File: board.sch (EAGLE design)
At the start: 75 parts, among them IC1 LM1117, J1 LHBEAMOUT, J10 ATEMP, J11 HORNOUT, J12 12V_SUPPLY, J13 STOPOUT, J14 TURNOUT, J15 FANOUT, J16 BLIGHTOUT, J17 AUXOUT, J18 AUX, J19 CAN, J2 BATT, J3 BLIGHT, J4 LHBEAM, J5 LRTURN, J6 WARNING, J7 HORN, J8 BREAK, J9 ABREAK, Q1 IRF7465TR, Q2 IRF7465TR, Q3 IRF7465TR, Q4 IRLML9301TRPBF, Q5 IRLML9301TRPBF, Q6 IRF7424TRPBF, Q7 IRF7424TRPBF, Q8 IRF7424TRPBF, Q9 IRLML9301TRPBF, U1 VOM1271T, U2 VOM1271T, U3 VOM1271T, U4 MC14504BDR2G, U5 MAX3051ESA+T

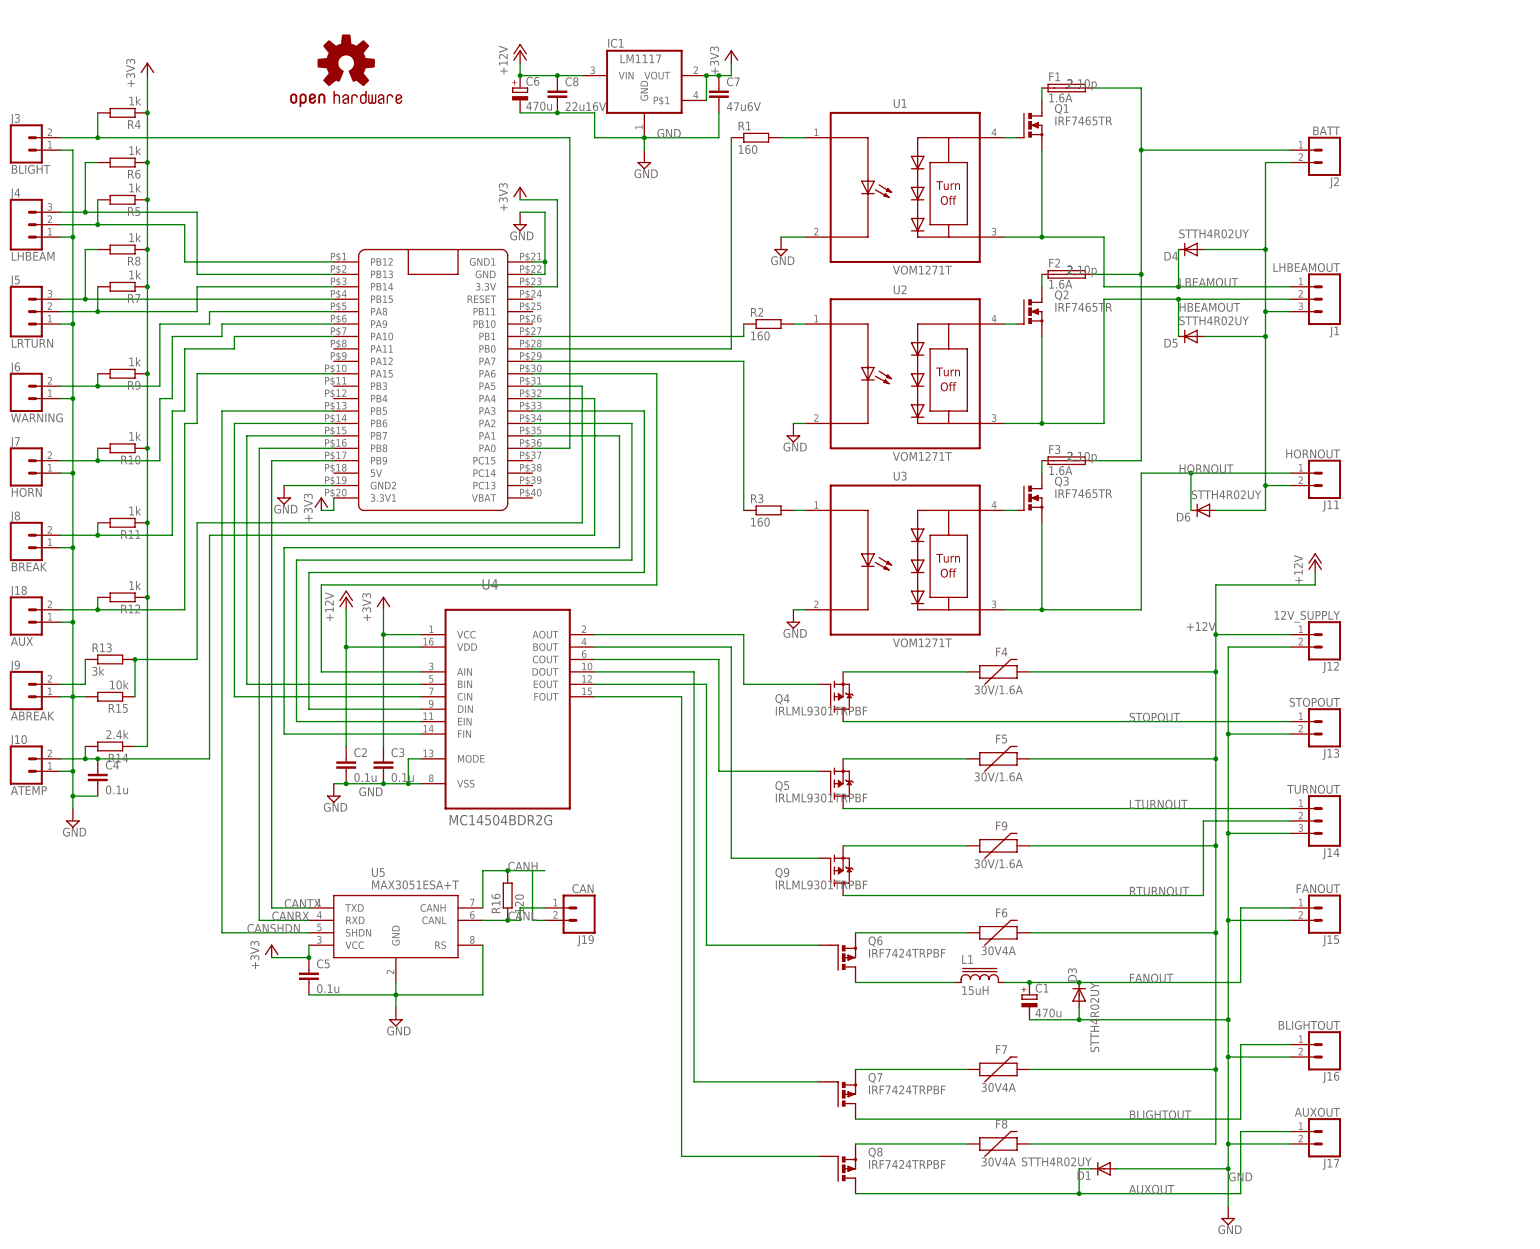
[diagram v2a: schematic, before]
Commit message: WIP
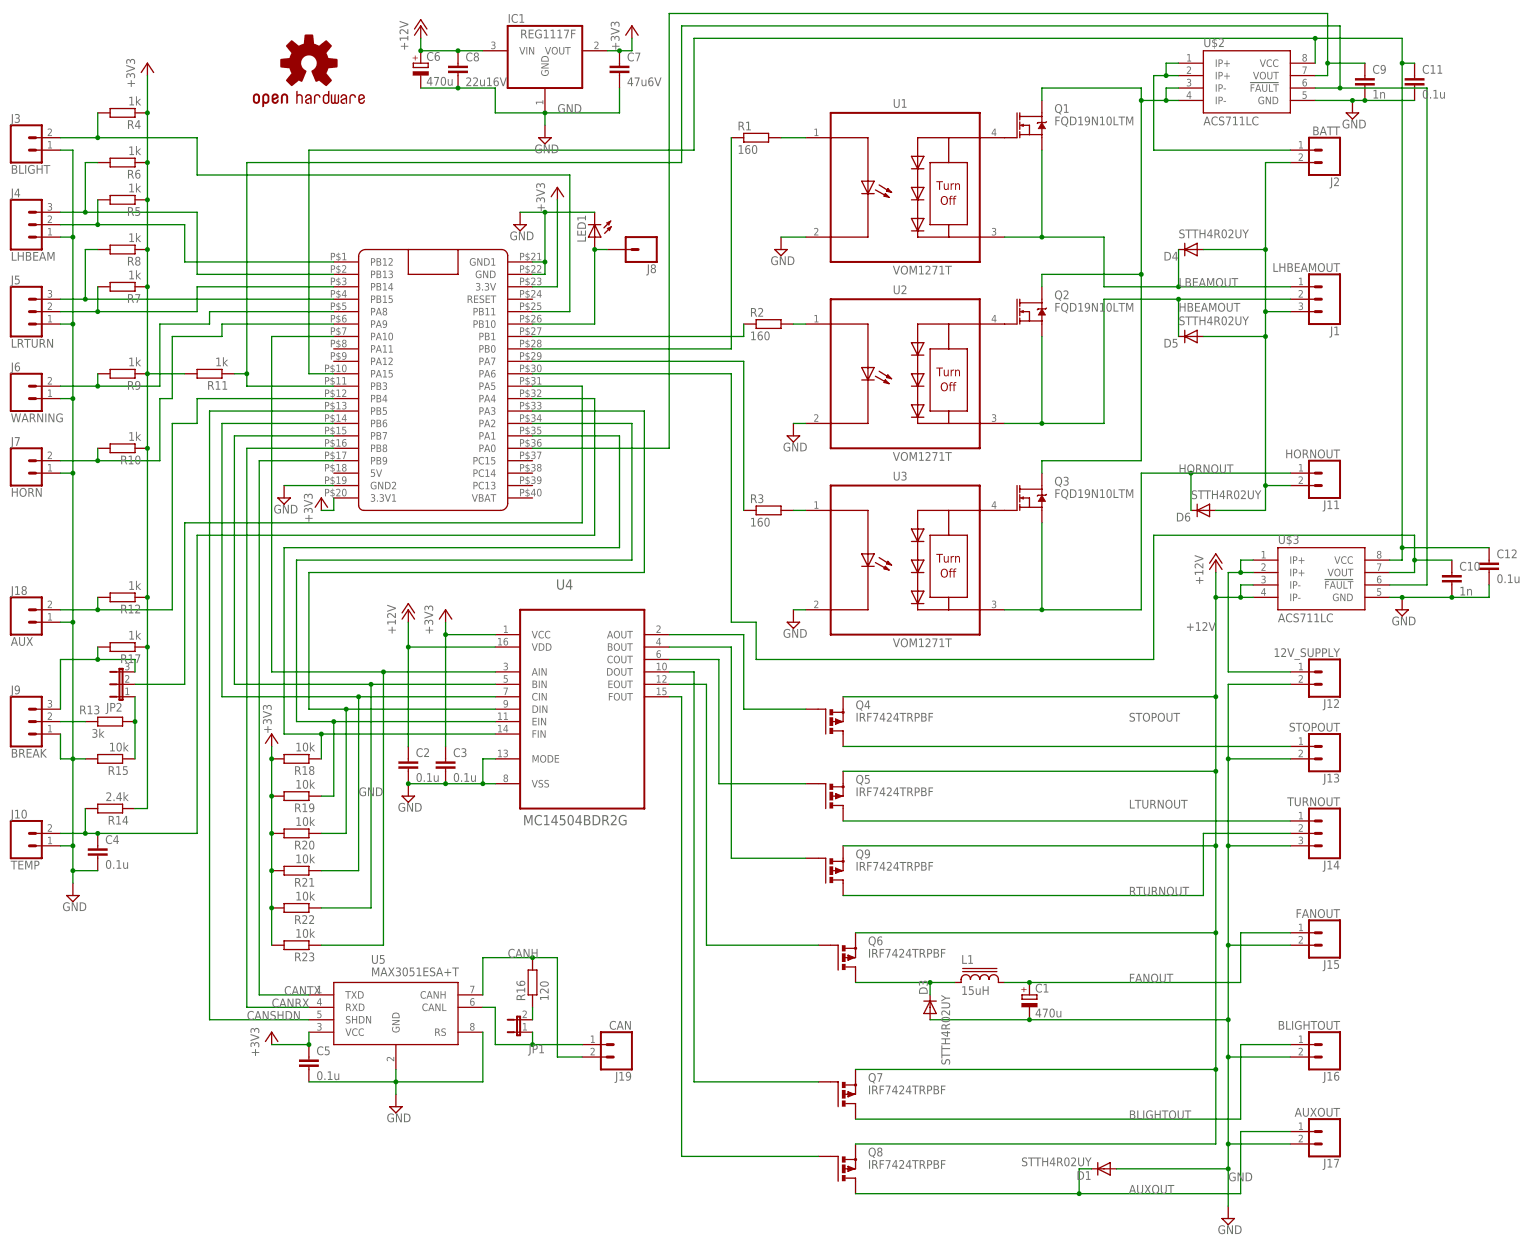
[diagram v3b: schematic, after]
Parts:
- removed F1, F2, F3: 1.6A, fuse:SHK20L
- removed F4, F5, F9: 30V/1.6A, SparkFun-Fuses:PPTC_PTH
- removed F6, F7, F8: 30V4A, svetozar:PPTC_WIDE
- added C10, C9: 1n, rcl:C-EUC0805
- added C11, C12: 0.1u, rcl:C-EUC0805
- added JP1: (no value), jumper:JP1E
- added JP2: (no value), jumper:JP2E
- added LED1: (no value), led:LEDSML0805
- added R17: 1k, rcl:R-EU_R0603
- added R18, R19, R20, R21, R22, R23: 10k, rcl:R-EU_R0603
- added U$2, U$3: ACS711LC, svetozar:ACS711
- C1, C6: device rcl:CPOL-EUE3.5-8 -> rcl:CPOL-EUF
- IC1: value LM1117 -> REG1117F; device svetozar:LM1117 -> burr-brown:REG1117F
- J10: value ATEMP -> TEMP
- J8: value BREAK -> (none); device SparkFun-Connectors:CONN_023.5MM -> SparkFun-Connectors:CONN_01; MPN DG350-3.5-02P-14-00AH -> (none); PRICE 5,80р -> (none); SHOP https://www.terraelectronica.ru/product/1115132 -> (none)
- J9: value ABREAK -> BREAK; device SparkFun-Connectors:CONN_023.5MM -> SparkFun-Connectors:CONN_03SCREW
- Q1, Q2, Q3: value IRF7465TR -> FQD19N10LTM; device transistor-power:N-MOSFET-SO8S -> SparkFun-DiscreteSemi:MOSFET-NCH-FDD8780; MPN IRF7465TRPBF -> FQD19N10LTM; PRICE 26,30р -> 15,80р; SHOP https://www.terraelectronica.ru/product/507651 -> https://www.terraelectronica.ru/product/675613
- Q4: value IRLML9301TRPBF -> IRF7424TRPBF; device svetozar:IRLML9301TRPBF -> transistor-power:P-MOSFET-SO8
- Q5, Q9: value IRLML9301TRPBF -> IRF7424TRPBF; device my:IRLML9301TRPBF -> transistor-power:P-MOSFET-SO8
- R10, R12, R13, R14, R15, R4, R5, R6, R7, R8, R9: device rcl:R-EU_R0805 -> rcl:R-EU_R0603
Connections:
- net ABRK renamed N$5
- removed net CANL: J19.1, R16.1, U5.CANL
- removed net HV1: F1.1A, Q1.D
- removed net HV2: F2.1A, Q2.D
- removed net HV3: F3.1A, Q3.D
- removed net N$15: J3.2, R4.2, U$1.PA0
- removed net N$16: F4.1, Q4.S
- removed net N$18: F5.1, Q5.S
- removed net N$19: F6.1, Q6.S
- removed net N$21: F7.1, Q7.S
- removed net N$22: F8.1, Q8.S
- removed net N$23: F9.1, Q9.S
- removed net N$34: J8.2, R11.2, U$1.PA10
- removed net N$36: J18.2, R12.2, U$1.PA15
- new net BATT+IN: J2.1, U$2.IP+@1, U$2.IP+@2
- new net CSENS1: C9.1, U$1.PA0, U$2.VOUT
- new net FAULT: R11.1, U$1.PB3, U$2.!FAULT, U$3.!FAULT
- new net IAUX: J18.2, R12.2, U$1.PB4
- new net IBLGHT: J3.2, R4.2, U$1.PB11
- new net N$1: JP1.2, R16.1
- new net N$2: J19.1, JP1.1, U5.CANL
- new net N$3: JP2.1, R13.2, R15.1
- new net N$4: J9.3, JP2.3, R17.2
- new net N$6: J8.1, LED1.A, U$1.PB10
- new net N$7: J12.1, U$3.IP+@1, U$3.IP+@2
- new net N$8: C10.1, U$1.PA6, U$3.VOUT
- new net N$9: C11.1, C12.1, U$1.PA15, U$2.VCC, U$3.VCC
- net +12V: now also Q4.S, Q5.S, Q6.S, Q7.S, Q8.S, Q9.S, U$3.IP-@3, U$3.IP-@4; no longer F4.2, F5.2, F6.2, F7.2, F8.2, F9.2, J12.1
- net +3V3: now also R11.2, R17.1, R18.2, R19.2, R20.2, R21.2, R22.2, R23.2; no longer IC1.P$1, R11.1
- net ABRK_S: now also JP2.2; no longer R13.2, R15.1
- net BATT+: now also Q1.D, Q2.D, Q3.D, U$2.IP-@3, U$2.IP-@4; no longer F1.2A, F2.2A, F3.2A, J2.1
- net FANOUT: no longer D3.C
- net GND: now also C10.2, C11.2, C12.2, C9.2, LED1.C, U$2.GND, U$3.GND; no longer J8.1
- net LVCTL1: now also R23.1, U$1.PA10; no longer U$1.PA6
- net LVCTL2: now also R22.1
- net LVCTL3: now also R21.1
- net LVCTL4: now also R20.1
- net LVCTL5: now also R19.1
- net LVCTL6: now also R18.1
- net N$17: now also D3.C
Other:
- moved on the sheet: C2, C3, C4, C5, C6, C7, C8, D3, J10, J12, J13, J14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
